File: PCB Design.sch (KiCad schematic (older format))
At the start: 112 parts, among them SW1 SW_Push, U1 ATmega32U4-AU, Y1 16MHz

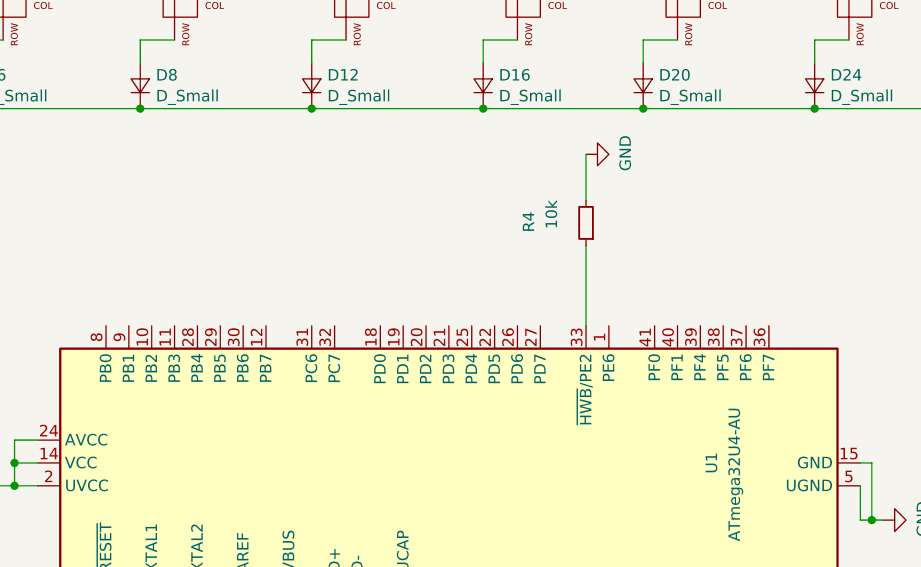
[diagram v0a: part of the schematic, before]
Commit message: Finished routing
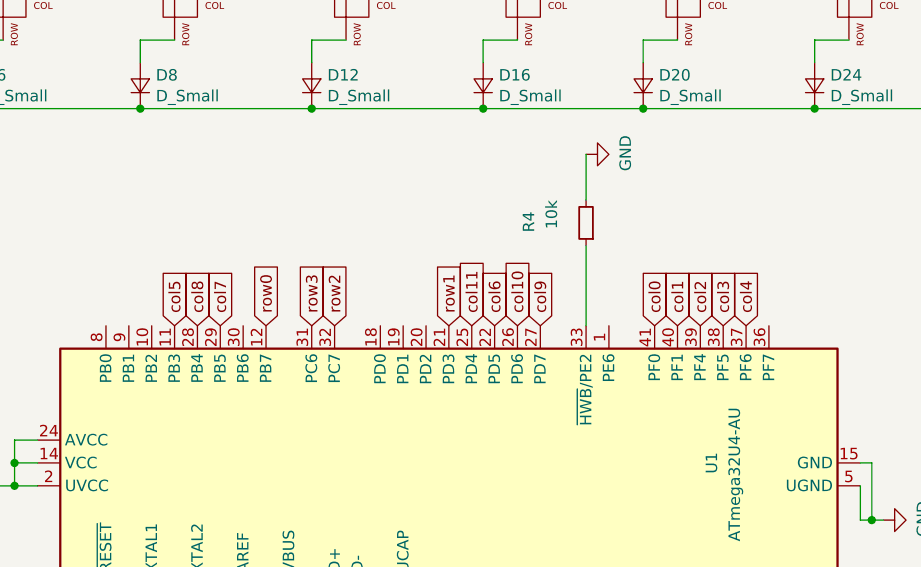
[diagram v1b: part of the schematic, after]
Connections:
- net col0: now also U1.41 (PF0)
- net col1: now also U1.40 (PF1)
- net col10: now also U1.26 (PD6)
- net col11: now also U1.25 (PD4)
- net col2: now also U1.39 (PF4)
- net col3: now also U1.38 (PF5)
- net col4: now also U1.37 (PF6)
- net col5: now also U1.11 (PB3)
- net col6: now also U1.22 (PD5)
- net col7: now also U1.29 (PB5)
- net col8: now also U1.28 (PB4)
- net col9: now also U1.27 (PD7)
- net row0: now also U1.12 (PB7)
- net row1: now also U1.21 (PD3)
- net row2: now also U1.32 (PC7)
- net row3: now also U1.31 (PC6)
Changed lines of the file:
@@
 	6200 4000 6900 4000
 Connection ~ 6200 4000
+Text GLabel 3300 4950 1    50   Input ~ 0
+col6
+Text GLabel 3100 4950 1    50   Input ~ 0
+row1
+Text GLabel 2300 4950 1    50   Input ~ 0
+row0
+Text GLabel 1900 4950 1    50   Input ~ 0
+col5
+Text GLabel 3200 4950 1    50   Input ~ 0
+col11
+Text GLabel 3400 4950 1    50   Input ~ 0
+col10
+Text GLabel 3500 4950 1    50   Input ~ 0
+col9
+Text GLabel 2000 4950 1    50   Input ~ 0
+col8
+Text GLabel 2100 4950 1    50   Input ~ 0
+col7
+Text GLabel 2500 4950 1    50   Input ~ 0
+row3
+Text GLabel 2600 4950 1    50   Input ~ 0
+row2
+Text GLabel 4000 4950 1    50   Input ~ 0
+col0
+Text GLabel 4100 4950 1    50   Input ~ 0
+col1
+Text GLabel 4200 4950 1    50   Input ~ 0
+col2
+Text GLabel 4300 4950 1    50   Input ~ 0
+col3
+Text GLabel 4400 4950 1    50   Input ~ 0
+col4
 $EndSCHEMATC
